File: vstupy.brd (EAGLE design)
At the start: 100 x 80 mm, 43 parts, among them IC1 4012N, IC2 4012N, IC3 4075N

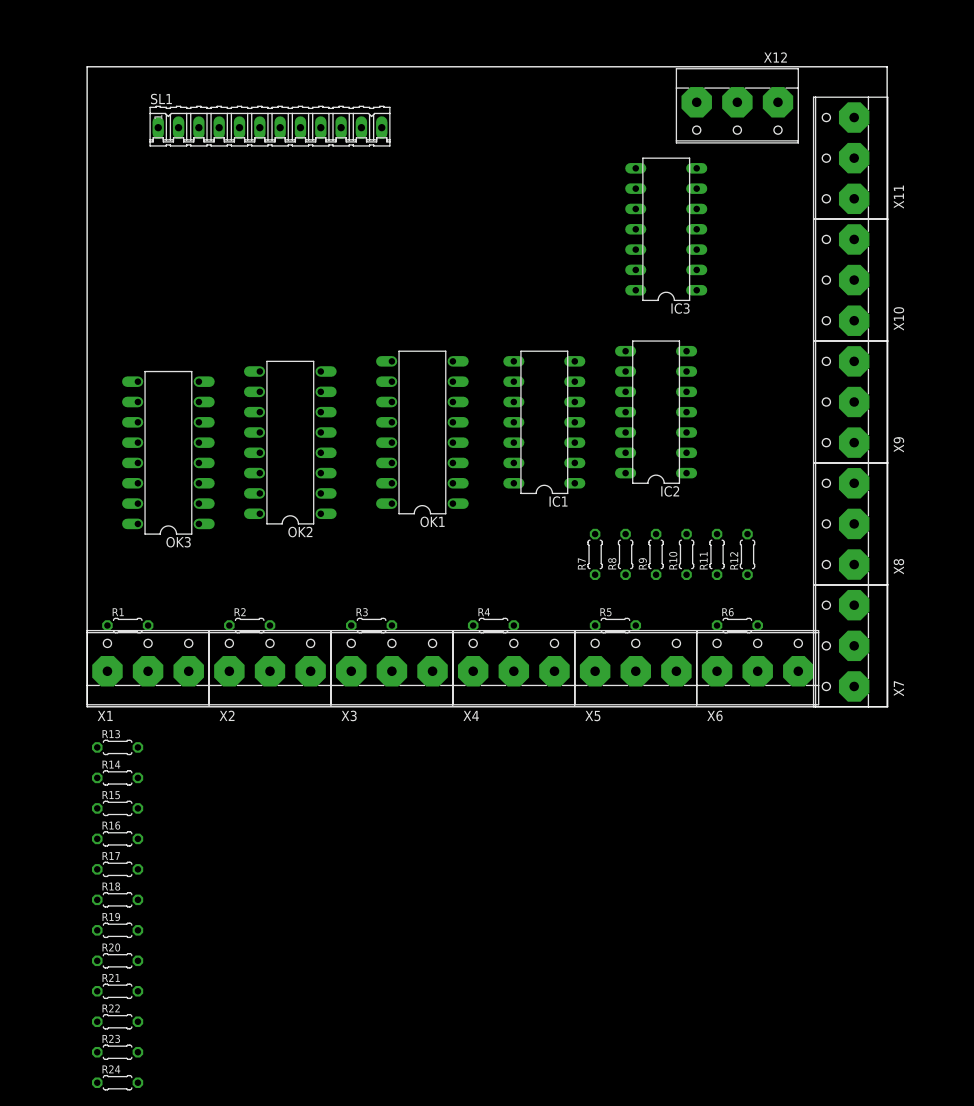
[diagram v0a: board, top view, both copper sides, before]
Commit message: uprava desky
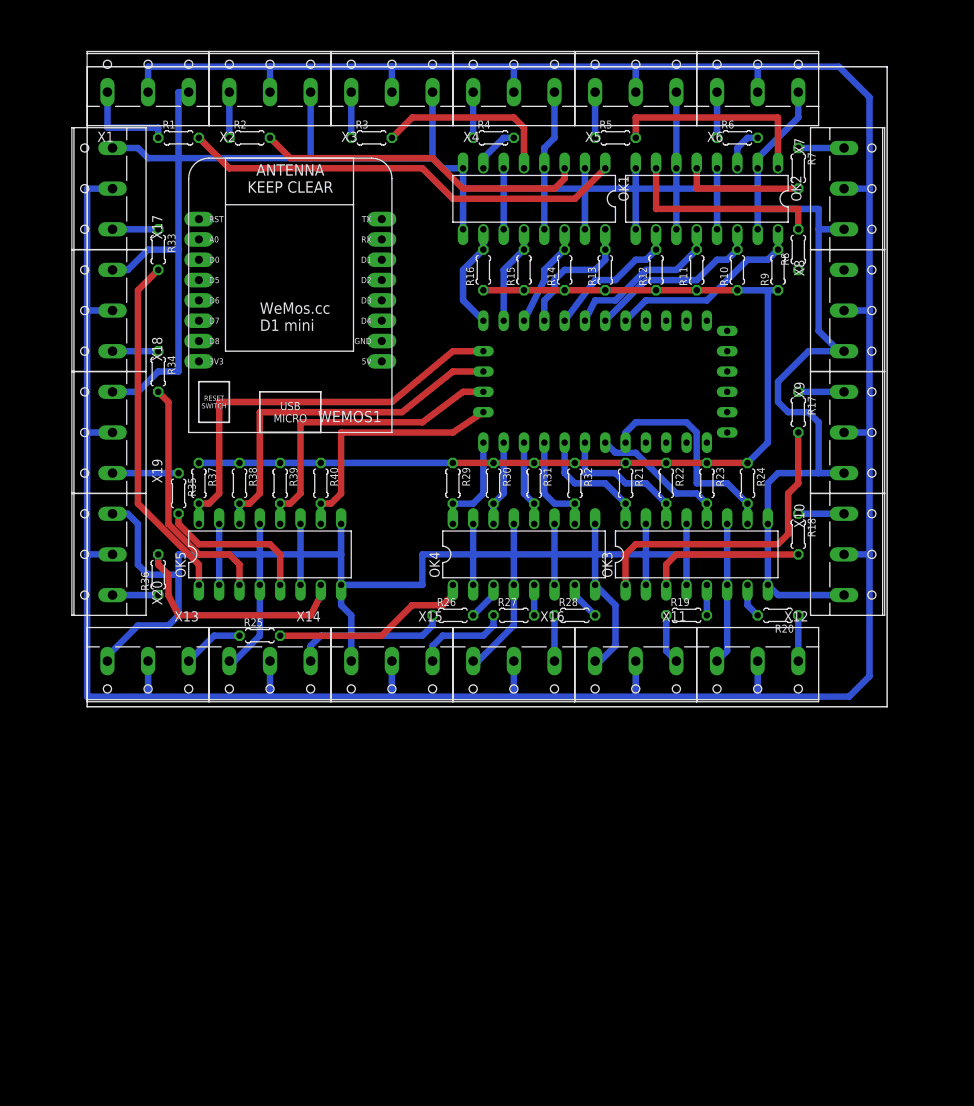
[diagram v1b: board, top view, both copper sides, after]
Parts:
- removed IC1, IC2: 4012N, 40xx:DIL14
- removed IC3: 4075N, 40xx:DIL14
- removed SL1: (no value), con-amp-quick:12P
- added OK4, OK5: PC847, optocoupler:DIL16
- added R25, R26, R27, R28, R29, R30, R31, R32, R33, R34, R35, R36, R37, R38, R39, R40: (no value), resistor:0204/5
- added U$1: PRO-MINI, Arduino-clone:PRO-MINI
- added WEMOS1: (no value), esp8266modules:WEMOS-D1-MINI
- added X13, X14, X15, X16, X17, X18, X19, X20: (no value), con-wago-508:W237-3E
- moved R24 108.7 mm to (82.5, 27.9), turned to 270 degrees
- moved R17 102.5 mm to (88.9, 36.8), turned to 270 degrees
- moved R23 102.4 mm to (77.5, 27.9), turned to 270 degrees
- moved R18 96.6 mm to (88.9, 21.6), turned to 270 degrees
- moved R22 96.1 mm to (72.4, 27.9), turned to 270 degrees
- moved R20 93.2 mm to (86.4, 11.4), turned to 180 degrees
- moved R21 89.8 mm to (67.3, 27.9), turned to 270 degrees
- moved R13 85.3 mm to (64.8, 54.6), turned to 90 degrees
- moved R14 84.6 mm to (59.7, 54.6), turned to 90 degrees
- moved R16 84.5 mm to (49.5, 54.6), turned to 90 degrees
- moved R15 84.3 mm to (54.6, 54.6), turned to 90 degrees
- moved R19 81.3 mm to (74.9, 11.4)
- moved X1 72.4 mm to (7.62, 77.5)
- moved X2 72.4 mm to (22.9, 77.5)
- moved X3 72.4 mm to (38.1, 77.5)
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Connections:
- removed net +5V: R13.1, R14.1, R15.1, R16.1, R17.1, R18.1, R19.1, R20.1, R21.1, R22.1, R23.1, R24.1
- removed net N$10 (its old number): OK3.3, R10.2
- removed net N$11 (its old number): OK3.5, R11.2
- removed net N$12 (its old number): OK3.7, R12.2
- removed net N$46: IC2.2, OK3.16, R21.2, SL1.9
- removed net N$9 (its old number): OK3.1, R9.2
- removed net VDD: IC1.14, IC2.14, IC3.14
- removed net VSS: IC1.7, IC2.7, IC3.7
- new net +3V3: R10.1, R11.1, R12.1, R13.1, R14.1, R15.1, R16.1, R21.1, R22.1, R23.1, R24.1, R29.1, R30.1, R31.1, R32.1, R37.1, R38.1, R39.1, R40.1, R9.1
- new net N$17: OK2.16, R9.2, U$1.D2
- new net N$18: OK2.14, R10.2, U$1.D3
- new net N$19: OK2.12, R11.2, U$1.D4
- new net N$20: OK2.10, R12.2, U$1.D5
- new net N$31: OK1.16, R13.2, U$1.D6
- new net N$32: OK1.14, R14.2, U$1.D7
- new net N$33: OK3.12, R23.2, U$1.A2
- new net N$34: OK1.12, R15.2, U$1.D8
- new net N$35: OK1.10, R16.2, U$1.D9
- new net N$36: OK3.10, R24.2, U$1.A3
- new net N$37: OK4.1, R25.2
- new net N$51: OK5.5, R35.2
- new net N$52: OK5.7, R36.2
- new net N$53: R33.1, X17.1
- new net N$54: R34.1, X18.1
- new net N$55: R35.1, X19.1
- new net N$56: R36.1, X20.1
- new net N$57: OK5.16, R37.2, U$1.A4
- new net N$58: OK5.14, R38.2, U$1.A5
- new net N$59: OK5.12, R39.2, U$1.A6
- new net N$60: OK5.10, R40.2, U$1.A7
- new net N$61: OK4.14, R30.2, U$1.D11
- new net RAW: U$1.RAW
- net +12V: now also X13.2, X14.2, X15.2, X16.2, X17.2, X18.2, X19.2, X20.2
- net GND: now also OK2.15, OK4.11, OK4.13, OK4.15, OK4.2, OK4.4, OK4.6, OK4.8, OK4.9, OK5.11, OK5.13, OK5.15, OK5.2, OK5.4, OK5.6, OK5.8, OK5.9, X13.3, X14.3, X15.3, X16.3, X17.3, X18.3, X19.3, X20.3
- net N$21: now also OK3.1, R17.2; no longer R9.1, X9.1
- net N$22: now also OK3.3, R18.2; no longer R10.1, X10.1
- net N$23: now also OK3.5, R19.2; no longer R11.1, X11.1
- net N$24: now also OK3.7, R20.2; no longer R12.1, X12.1
- net N$25: now also R17.1, X9.1; no longer IC1.1, IC3.1, IC3.2, IC3.8
- net N$26: now also R18.1, X10.1; no longer IC1.13, IC3.3, IC3.4, IC3.5
- net N$27: now also R19.1, X11.1; no longer IC2.1, IC3.11, IC3.12, IC3.13
- net N$28: now also R20.1, X12.1; no longer IC2.9, IC3.9
- net N$29: now also OK3.16, R21.2, U$1.A0; no longer IC2.10, IC3.6
- net N$30: now also OK3.14, R22.2, U$1.A1; no longer IC2.11, IC2.12, IC3.10
- net N$38: now also OK4.3, R26.2; no longer IC1.2, OK1.16, R13.2, SL1.1
- net N$39: now also OK4.5, R27.2; no longer IC1.3, OK1.14, R14.2, SL1.2
- net N$40: now also OK4.7, R28.2; no longer IC1.4, OK1.12, R15.2, SL1.3
- net N$41: now also R25.1, X13.1; no longer IC1.5, OK1.10, R16.2, SL1.4
- net N$42: now also R26.1, X14.1; no longer IC1.9, OK2.16, R17.2, SL1.5
- net N$43: now also R27.1, X15.1; no longer IC1.10, OK2.14, R18.2, SL1.6
- net N$44: now also R28.1, X16.1; no longer IC1.11, OK2.12, R19.2, SL1.7
- net N$45: now also OK4.16, R29.2, U$1.D10; no longer IC1.12, OK2.10, R20.2, SL1.8
- net N$47: now also OK4.12, R31.2, U$1.D12; no longer IC2.3, OK3.14, R22.2, SL1.10
- net N$48: now also OK4.10, R32.2, U$1.D13; no longer IC2.4, OK3.12, R23.2, SL1.11
- net N$49: now also OK5.1, R33.2; no longer IC2.5, OK3.10, R24.2, SL1.12
- net N$50: now also OK5.3, R34.2; no longer OK2.15
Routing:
- net GND: track 0.00 -> 584.5 mm
- net +12V: track 0.00 -> 398.2 mm
- net +3V3: track 0.00 -> 128.1 mm
- net N$1: track 0.00 -> 55.5 mm
- net N$57: track 0.00 -> 52.4 mm
- net N$58: track 0.00 -> 45.5 mm
- net N$49: track 0.00 -> 43.6 mm
- net N$2: track 0.00 -> 41.3 mm
- net N$59: track 0.00 -> 38.6 mm
- net N$21: track 0.00 -> 38.4 mm
- net N$60: track 0.00 -> 31.8 mm
- net N$50: track 0.00 -> 30.6 mm
- net N$52: track 0.00 -> 29.1 mm
- net N$36: track 0.00 -> 27.5 mm
- net N$5: track 0.00 -> 26.7 mm
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
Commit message: +
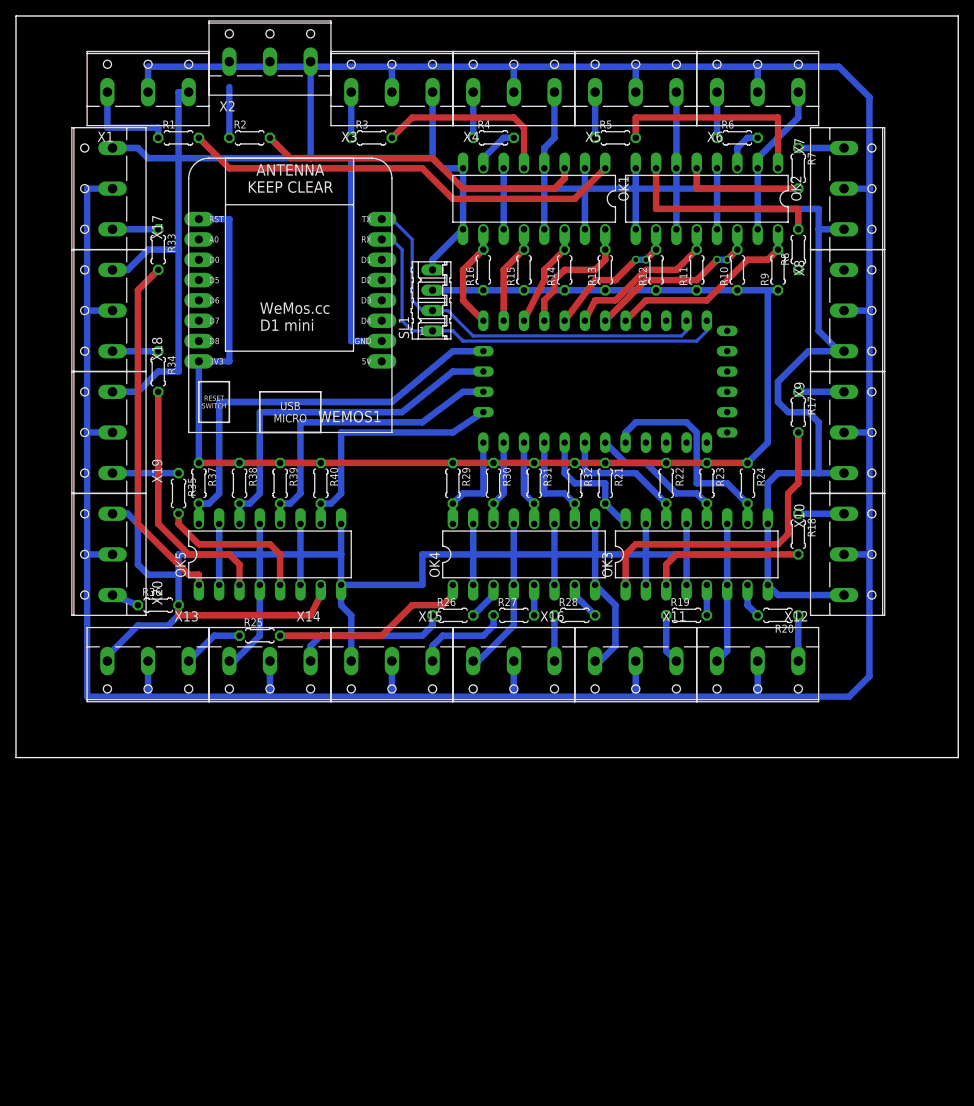
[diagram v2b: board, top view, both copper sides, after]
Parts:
- added SL1: (no value), con-amp-quick:04P
- moved R36 3.81 mm to (8.89, 12.7), turned to 0 degrees
- moved X2 3.81 mm to (22.9, 81.3)
- moved R21 2.54 mm to (64.8, 27.9)
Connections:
- removed net RAW: U$1.RAW
- new net N$46: SL1.1, U$1.TX0, WEMOS1.RX
- new net N$62: SL1.2, U$1.RX1, WEMOS1.TX
- net +3V3: now also SL1.3, U$1.RAW, WEMOS1.3V3, WEMOS1.RESET
- net GND: now also SL1.4, U$1.GND, WEMOS1.GND
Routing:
- net N$46: track 0.00 -> 52.9 mm
- net N$62: track 0.00 -> 50.1 mm
- net +3V3: track 128.1 -> 172.5 mm
- net GND: track 584.5 -> 621.6 mm
- net N$52: track 29.1 -> 21.9 mm
- net +12V: track 398.2 -> 395.7 mm
- net N$56: track 5.72 -> 3.42 mm
- net N$50: track 30.6 -> 31.3 mm
- net N$49: track 43.6 -> 44.3 mm
- net N$20: vias 0 -> 2
- net N$18: vias 0 -> 2
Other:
- board size 100 x 80 mm -> 117.8 x 92.7 mm

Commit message: uprava desky
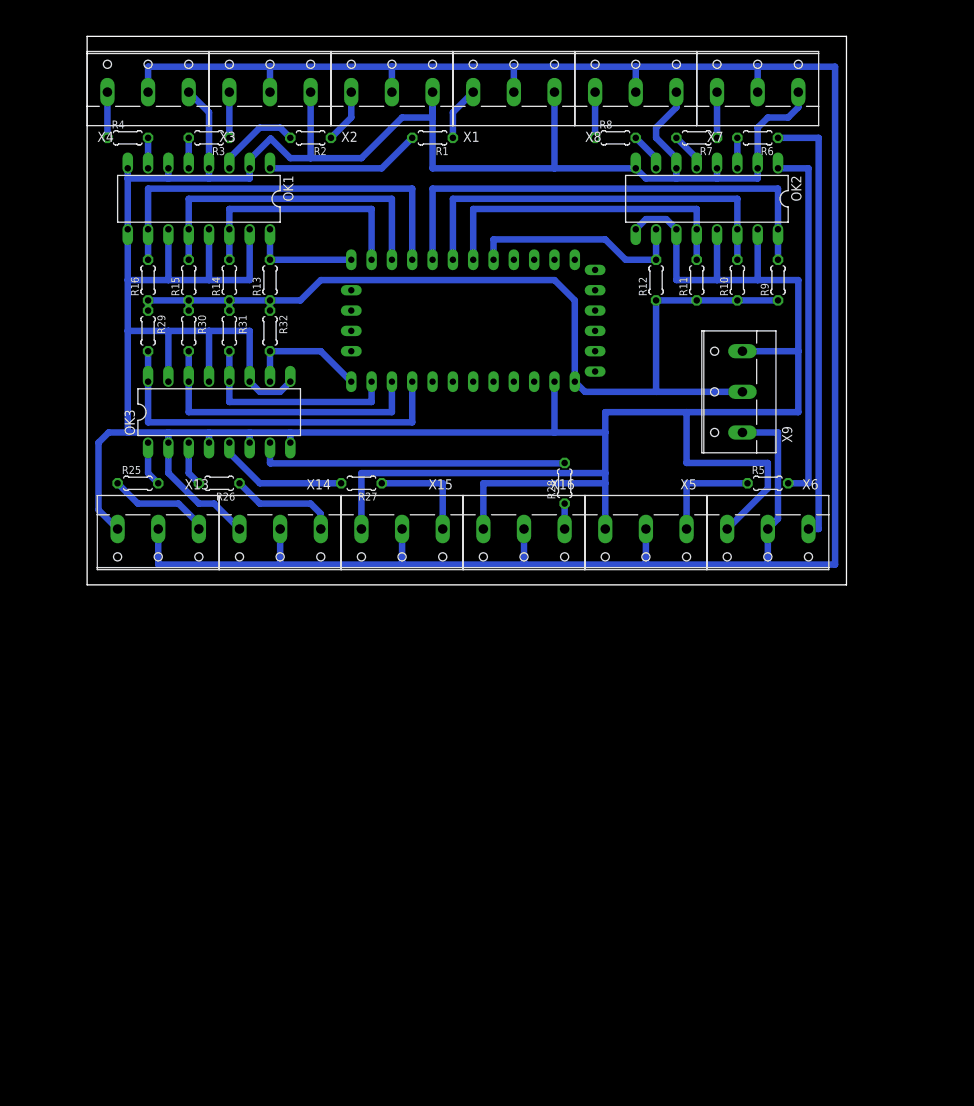
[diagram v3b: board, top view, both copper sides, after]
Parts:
- removed OK4, OK5: PC847, optocoupler:DIL16
- removed R17, R18, R19, R20, R21, R22, R23, R24, R33, R34, R35, R36, R37, R38, R39, R40: (no value), resistor:0204/5
- removed SL1: (no value), con-amp-quick:04P
- removed WEMOS1: (no value), esp8266modules:WEMOS-D1-MINI
- removed X10, X11, X12, X17, X18, X19, X20: (no value), con-wago-508:W237-3E
- moved OK3 62.3 mm to (16.5, 36.8)
- moved X5 55.9 mm to (69.8, 21.6), turned to 180 degrees
- moved X6 55.9 mm to (85.1, 21.6), turned to 180 degrees
- moved R5 47.2 mm to (85.1, 27.9)
- moved X1 45.7 mm to (53.3, 77.5)
- moved X4 45.7 mm to (7.62, 77.5)
- moved R4 45.7 mm to (5.08, 71.1)
- moved R29 42.6 mm to (7.62, 47.0)
- moved R31 42.6 mm to (17.8, 47.0)
- moved R32 42.6 mm to (22.9, 47.0)
- moved R30 42.6 mm to (12.7, 47.0)
- moved R16 41.9 mm to (7.62, 53.3)
- moved R13 41.9 mm to (22.9, 53.3)
- moved R14 41.9 mm to (17.8, 53.3)
- moved R15 41.9 mm to (12.7, 53.3)
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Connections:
- removed net +3V3: R10.1, R11.1, R12.1, R13.1, R14.1, R15.1, R16.1, R21.1, R22.1, R23.1, R24.1, R29.1, R30.1, R31.1, R32.1, R37.1, R38.1, R39.1, R40.1, R9.1, SL1.3, U$1.RAW, WEMOS1.3V3, WEMOS1.RESET
- removed net N$24: OK3.7, R20.2
- removed net N$25: R17.1, X9.1
- removed net N$26: R18.1, X10.1
- removed net N$27: R19.1, X11.1
- removed net N$28: R20.1, X12.1
- removed net N$29: OK3.16, R21.2, U$1.A0
- removed net N$30: OK3.14, R22.2, U$1.A1
- removed net N$31: OK1.16, R13.2, U$1.D6
- removed net N$32: OK1.14, R14.2, U$1.D7
- removed net N$33: OK3.12, R23.2, U$1.A2
- removed net N$34: OK1.12, R15.2, U$1.D8
- removed net N$36: OK3.10, R24.2, U$1.A3
- removed net N$46: SL1.1, U$1.TX0, WEMOS1.RX
- removed net N$49: OK5.1, R33.2
- removed net N$50: OK5.3, R34.2
- removed net N$51: OK5.5, R35.2
- removed net N$52: OK5.7, R36.2
- removed net N$53: R33.1, X17.1
- removed net N$54: R34.1, X18.1
- removed net N$55: R35.1, X19.1
- removed net N$56: R36.1, X20.1
- removed net N$57: OK5.16, R37.2, U$1.A4
- removed net N$58: OK5.14, R38.2, U$1.A5
- removed net N$59: OK5.12, R39.2, U$1.A6
- removed net N$60: OK5.10, R40.2, U$1.A7
- removed net N$62: SL1.2, U$1.RX1, WEMOS1.TX
- new net +5V: R10.1, R11.1, R12.1, R13.1, R14.1, R15.1, R16.1, R29.1, R30.1, R31.1, R32.1, R9.1, U$1.RAW, X9.2
- net +12V: now also X9.1; no longer X10.2, X11.2, X12.2, X17.2, X18.2, X19.2, X20.2, X9.2
- net GND: no longer OK4.11, OK4.13, OK4.15, OK4.2, OK4.4, OK4.6, OK4.8, OK4.9, OK5.11, OK5.13, OK5.15, OK5.2, OK5.4, OK5.6, OK5.8, OK5.9, SL1.4, WEMOS1.GND, X10.3, X11.3, X12.3, X17.3, X18.3, X19.3, X20.3
- net N$17: now also U$1.D5; no longer U$1.D2
- net N$18: now also U$1.D4; no longer U$1.D3
- net N$19: now also U$1.D3; no longer U$1.D4
- net N$20: now also U$1.D2; no longer U$1.D5
- net N$21: now also OK1.16, R13.2, U$1.D9; no longer OK3.1, R17.2
- net N$22: now also OK1.14, R14.2, U$1.D8; no longer OK3.3, R18.2
- net N$23: now also OK1.12, R15.2, U$1.D7; no longer OK3.5, R19.2
- net N$35: now also U$1.D6; no longer U$1.D9
- net N$37: now also OK3.1; no longer OK4.1
- net N$38: now also OK3.3; no longer OK4.3
- net N$39: now also OK3.5; no longer OK4.5
- net N$40: now also OK3.7; no longer OK4.7
- net N$45: now also OK3.16, U$1.D13; no longer OK4.16, U$1.D10
- net N$47: now also OK3.12, U$1.D11; no longer OK4.12, U$1.D12
- net N$48: now also OK3.10, U$1.D10; no longer OK4.10, U$1.D13
- net N$61: now also OK3.14, U$1.D12; no longer OK4.14, U$1.D11
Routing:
- net +3V3: track 172.5 -> 0.00 mm
- net +5V: track 0.00 -> 118.8 mm
- net +12V: track 395.7 -> 296.1 mm
- net GND: track 621.6 -> 556.4 mm
- net N$46: track 52.9 -> 0.00 mm
- net N$57: track 52.4 -> 0.00 mm
- net N$62: track 50.1 -> 0.00 mm
- net N$10: track 5.71 -> 55.2 mm
- net N$58: track 45.5 -> 0.00 mm
- net N$49: track 44.3 -> 0.00 mm
- net N$59: track 38.6 -> 0.00 mm
- net N$35: track 13.5 -> 50.8 mm
- net N$23: track 3.81 -> 40.6 mm
- net N$1: track 55.5 -> 19.4 mm
- net N$17: track 25.3 -> 61.0 mm
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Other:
- board size 117.8 x 92.7 mm -> 94.9 x 68.6 mm
